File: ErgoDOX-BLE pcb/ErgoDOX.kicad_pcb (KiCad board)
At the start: 2 copper layers, 182.8 x 158.9 mm, 115 parts, among them J1 Conn_01x04, J2 Conn_01x02_Female, J3 Conn_01x02_Female, J4 Conn_01x02, J5 Conn_01x02, P1 USB_C_Plug_USB2.0, Q1 Q_NPN_BCE, SW0:10 SW0:3, SW0:11 SW0:2, SW0:12 SW0:1, SW0:7 SW0:6, SW0:8 SW0:5, SW0:9 SW0:4, SW1:10 SW1:3, SW1:11 SW1:2, SW1:12 SW1:1, SW1:13 SW1:0, SW1:9 SW1:4, SW2:10 SW2:3, SW2:11 SW2:2, SW2:12 SW2:1, SW2:13 SW2:0, SW2:7 SW2:6, SW2:8 SW2:5, SW2:9 SW2:4, SW3:10 SW3:3, SW3:11 SW3:2, SW3:12 SW3:1, SW3:13 SW3:0, SW3:8 SW3:5, SW3:9 SW3:4, SW4:10 SW4:3, SW4:11 SW4:2, SW4:12 SW4:1, SW4:13 SW4:0, SW4:7 SW4:6, SW4:8 SW4:5, SW4:9 SW4:4, SW5:10 SW5:3, SW5:11 SW5:2, SW5:12 SW5:1, SW5:13 SW5:0, SW5:7 SW5:6, SW5:8 SW5:5, SW5:9 SW5:4, U1 MCP23018, U3 C0720B001F

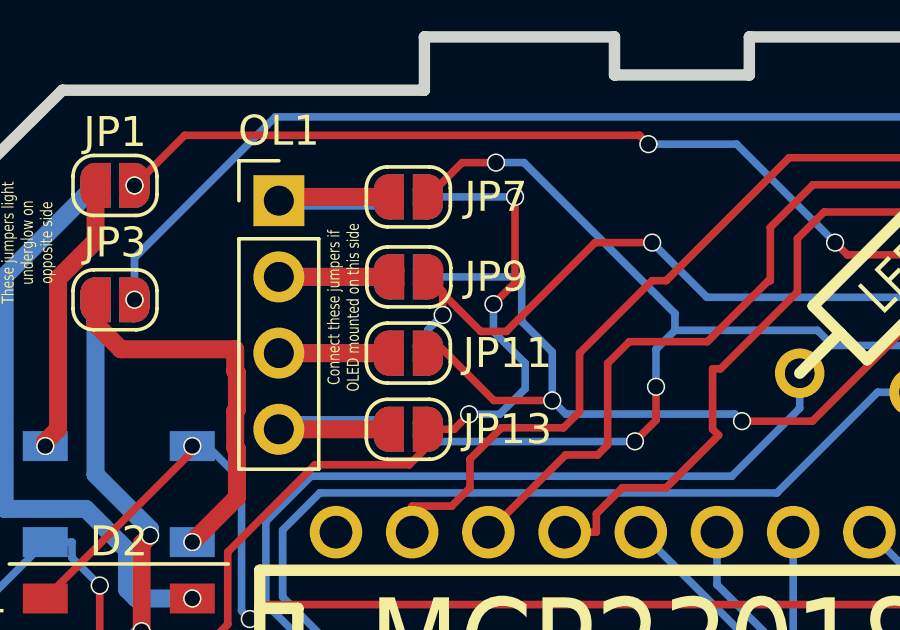
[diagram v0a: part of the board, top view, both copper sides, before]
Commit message: a touch more routing
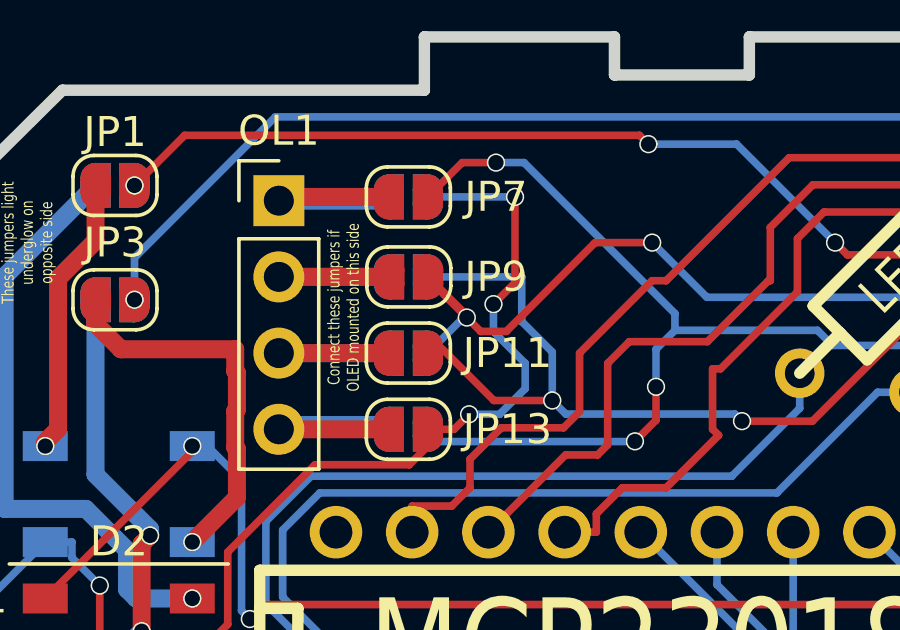
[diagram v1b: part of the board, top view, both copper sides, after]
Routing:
- net /SCL: track 179.6 -> 180.3 mm
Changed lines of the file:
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@@
   (segment (start 110.998 35.868796) (end 110.272102 35.142898) (width 0.254) (layer "F.Cu") (net 89))
   (segment (start 95.469144 39.918577) (end 95.631 39.756721) (width 0.254) (layer "F.Cu") (net 89))
+  (segment (start 79.291059 39.764059) (end 78.008 38.481) (width 0.254) (layer "F.Cu") (net 89))
   (segment (start 80.604789 40.299211) (end 83.566 37.338) (width 0.254) (layer "F.Cu") (net 89))
   (segment (start 94.791361 40.898506) (end 94.489215 40.898506) (width 0.254) (layer "F.Cu") (net 89))
@@
   (segment (start 196.469 54.102) (end 196.469 36.9765) (width 0.254) (layer "F.Cu") (net 89))
   (segment (start 116.586 45.085) (end 116.586 46.99) (width 0.254) (layer "F.Cu") (net 89))
-  (segment (start 78.486 39.751) (end 78.486 38.959) (width 0.254) (layer "F.Cu") (net 89))
   (segment (start 110.998 42.164) (end 110.998 35.868796) (width 0.254) (layer "F.Cu") (net 89))
   (segment (start 102.87 51.079444) (end 101.079278 49.288722) (width 0.254) (layer "F.Cu") (net 89))
@@
   (segment (start 78.486 39.029882) (end 79.755329 40.299211) (width 0.254) (layer "F.Cu") (net 89))
   (segment (start 97.028 44.86338) (end 95.627709 43.463089) (width 0.254) (layer "F.Cu") (net 89))
-  (segment (start 78.486 38.959) (end 78.008 38.481) (width 0.254) (layer "F.Cu") (net 89))
   (segment (start 121.285 51.689) (end 140.58445 51.689) (width 0.254) (layer "F.Cu") (net 89))
   (segment (start 111.2261 42.3921) (end 111.2261 47.0911) (width 0.254) (layer "F.Cu") (net 89))
+  (segment (start 79.291059 39.834941) (end 79.291059 39.764059) (width 0.254) (layer "F.Cu") (net 89))
   (via (at 101.079278 49.288722) (size 0.6096) (drill 0.508) (layers "F.Cu" "B.Cu") (net 89))
   (via (at 97.028 44.86338) (size 0.6096) (drill 0.508) (layers "F.Cu" "B.Cu") (net 89))
   (via (at 154.797969 53.705969) (size 0.6096) (drill 0.508) (layers "F.Cu" "B.Cu") (net 89))
   (via (at 196.469 45.974) (size 0.6096) (drill 0.508) (layers "F.Cu" "B.Cu") (net 89))
-  (via (at 78.486 39.751) (size 0.6096) (drill 0.508) (layers "F.Cu" "B.Cu") (net 89))
+  (via (at 79.291059 39.834941) (size 0.6096) (drill 0.508) (layers "F.Cu" "B.Cu") (net 89))
   (via (at 110.998 42.164) (size 0.6096) (drill 0.508) (layers "F.Cu" "B.Cu") (net 89))
   (via (at 116.586 45.085) (size 0.6096) (drill 0.508) (layers "F.Cu" "B.Cu") (net 89))
@@
   (segment (start 99.06 46.89538) (end 99.06 47.269443) (width 0.254) (layer "B.Cu") (net 89))
   (segment (start 95.040684 39.160684) (end 87.293684 39.160684) (width 0.254) (layer "B.Cu") (net 89))
-  (segment (start 77.993 41.021) (end 77.993 40.244) (width 0.254) (layer "B.Cu") (net 89))
   (segment (start 87.293684 39.160684) (end 85.471 37.338) (width 0.254) (layer "B.Cu") (net 89))
   (segment (start 108.92952 49.38768) (end 111.2261 47.0911) (width 0.254) (layer "B.Cu") (net 89))
@@
   (segment (start 99.06 47.269443) (end 101.178237 49.38768) (width 0.254) (layer "B.Cu") (net 89))
   (segment (start 114.427 42.164) (end 110.998 42.164) (width 0.254) (layer "B.Cu") (net 89))
+  (segment (start 79.291059 39.834941) (end 79.179059 39.834941) (width 0.254) (layer "B.Cu") (net 89))
   (segment (start 116.586 45.085) (end 115.42768 43.92668) (width 0.254) (layer "B.Cu") (net 89))
   (segment (start 115.42768 43.16468) (end 114.427 42.164) (width 0.254) (layer "B.Cu") (net 89))
   (segment (start 97.028 44.86338) (end 99.06 46.89538) (width 0.254) (layer "B.Cu") (net 89))
-  (segment (start 77.993 40.244) (end 78.486 39.751) (width 0.254) (layer "B.Cu") (net 89))
+  (segment (start 79.179059 39.834941) (end 77.993 41.021) (width 0.254) (layer "B.Cu") (net 89))
   (segment (start 133.35 143.51) (end 133.35 144.764311) (width 0.254) (layer "F.Cu") (net 90))
   (segment (start 133.35 106.664311) (end 133.992845 107.307156) (width 0.254) (layer "F.Cu") (net 90))
